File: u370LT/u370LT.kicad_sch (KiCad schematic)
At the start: 0 parts

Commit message: Updated northbridge more
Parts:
- added U1: ~, Library:BGA-676_26x26_35.0x35.0mm, symbol Library:VT82C694X
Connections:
- new net: U1.A1 (GND), U1.A14 (GND), U1.A26 (GND), U1.AA19 (GND), U1.AA21 (GND), U1.AA6 (GND), U1.AA8 (GND), U1.AB12 (GND), U1.AB15 (GND), U1.AB24 (GND), U1.AB25 (GND), U1.AC4 (GND), U1.AD18 (GND), U1.AD22 (GND), U1.AD9 (GND), U1.AE23 (GND), U1.AF1 (GND), U1.AF13 (GND), U1.AF26 (GND), U1.C18 (GND), U1.C22 (GND), U1.C5 (GND), U1.C9 (GND), U1.E12 (GND), U1.E15 (GND), U1.E24 (GND), U1.E3 (GND), U1.F19 (GND), U1.F21 (GND), U1.F6 (GND), U1.F8 (GND), U1.H21 (GND), U1.H6 (GND), U1.J24 (GND), U1.J3 (GND), U1.K1 (GND), U1.K7 (GND), U1.L12 (GND), U1.L15 (GND), U1.M11 (GND), U1.M13 (GND), U1.M14 (GND), U1.M16 (GND), U1.N12 (GND), U1.N13 (GND), U1.N14 (GND), U1.N15 (GND), U1.N24 (GND), U1.N7 (GND), U1.P12 (GND), U1.P13 (GND), U1.P14 (GND), U1.P15 (GND), U1.P22 (GND), U1.P26 (GND), U1.P3 (GND), U1.P7 (GND), U1.R11 (GND), U1.R13 (GND), U1.R14 (GND), U1.R16 (GND), U1.R22 (GND), U1.T12 (GND), U1.T15 (GND), U1.U6 (GND), U1.V24 (GND), U1.Y3 (GND), U1.Y6 (GND), U1.Y7 (GND), U1.Y8 (GND)
- new net: U1.AA18 (VCC), U1.AA20 (VCC), U1.AA9 (VCC), U1.AE26 (VCC), U1.AF14 (VCC), U1.B1 (VCC), U1.C2 (VCC), U1.F18 (VCC), U1.F20 (VCC), U1.F7 (VCC), U1.F9 (VCC), U1.G21 (VCC), U1.G6 (VCC), U1.J21 (VCC), U1.J6 (VCC), U1.L11 (VCC), U1.L13 (VCC), U1.L14 (VCC), U1.L16 (VCC), U1.M12 (VCC), U1.M15 (VCC), U1.N11 (VCC), U1.N16 (VCC), U1.N26 (VCC), U1.P11 (VCC), U1.P16 (VCC), U1.R12 (VCC), U1.R15 (VCC), U1.T11 (VCC), U1.T13 (VCC), U1.T14 (VCC), U1.T16 (VCC), U1.V21 (VCC)
- new net: U1.AA3 (VCCQ), U1.AA7 (VCCQ), U1.L6 (VCCQ), U1.L7 (VCCQ), U1.R3 (VCCQ), U1.R6 (VCCQ), U1.R7 (VCCQ)
- new net: U1.AD4 (VCCQQ), U1.W6 (VCCQ)
- new net: U1.L4 (ST0), U1.M4 (ST2)
- new net: U1.M21 (GNDA), U1.M22 (GNDA), U1.U7 (GNDA), U1.W21 (GNDA)
- new net: U1.N21 (VCCA), U1.N22 (VCCA), U1.V6 (VCCA), U1.Y21 (VCCA)

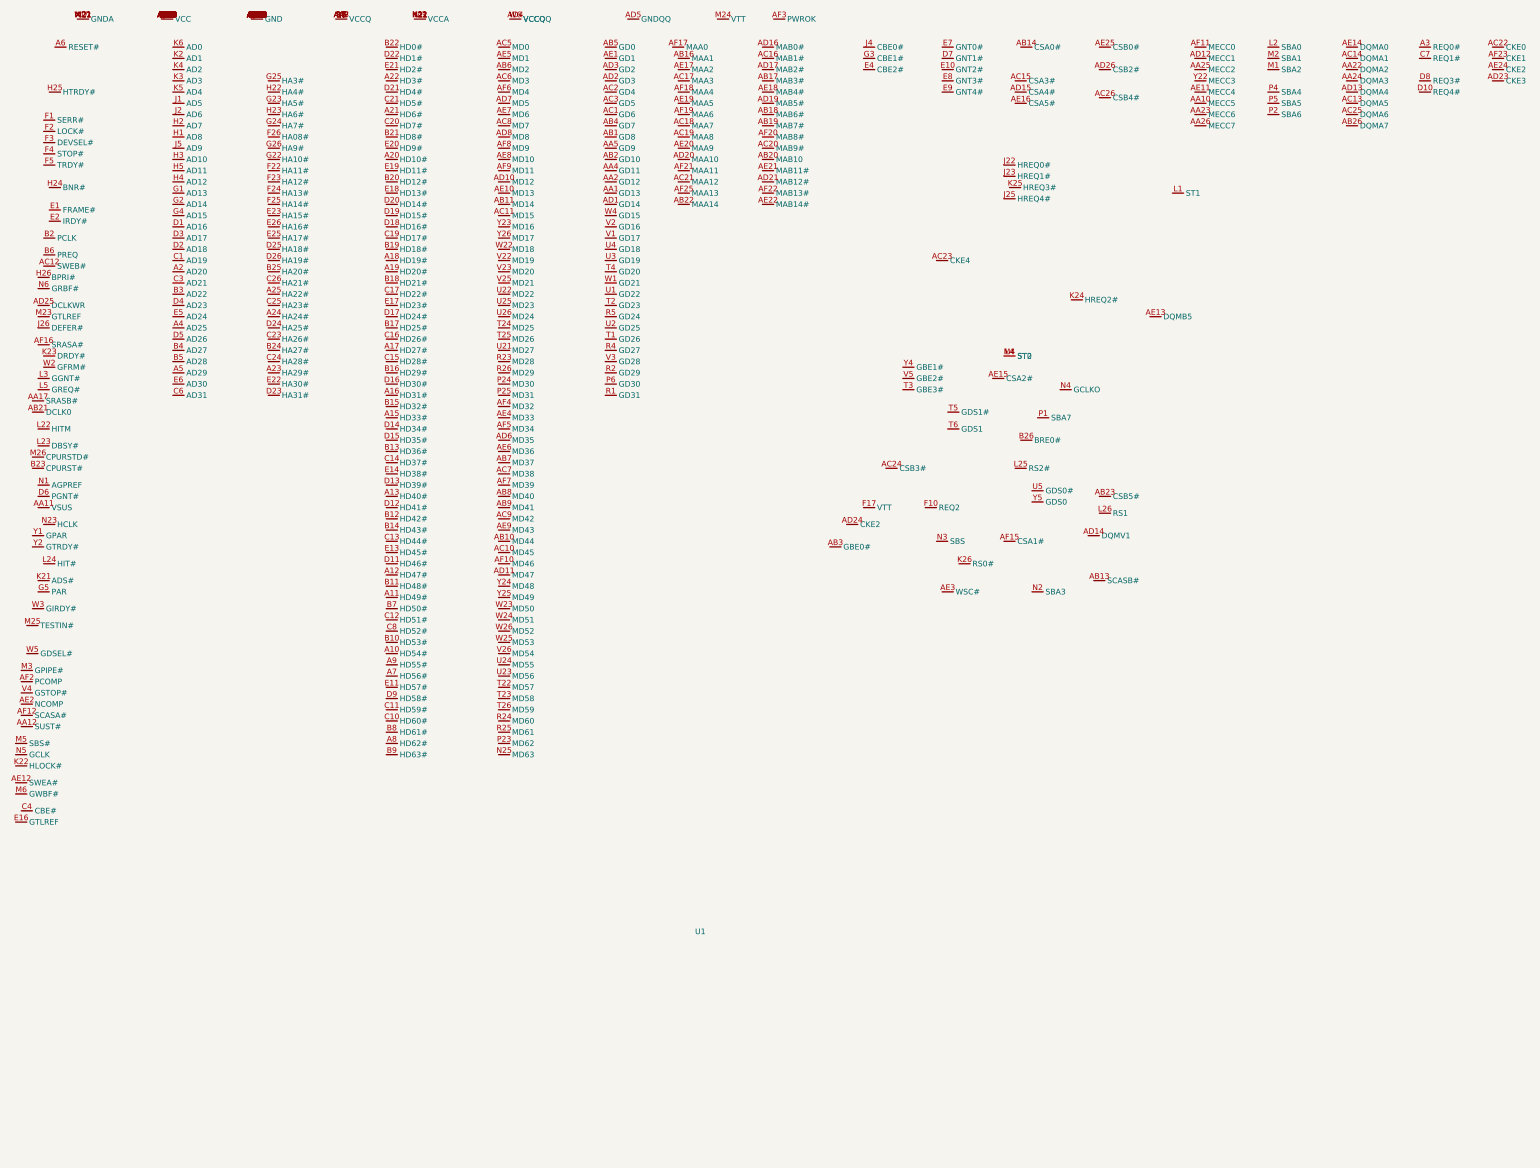
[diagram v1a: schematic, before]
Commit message: NB fixed up, SB started
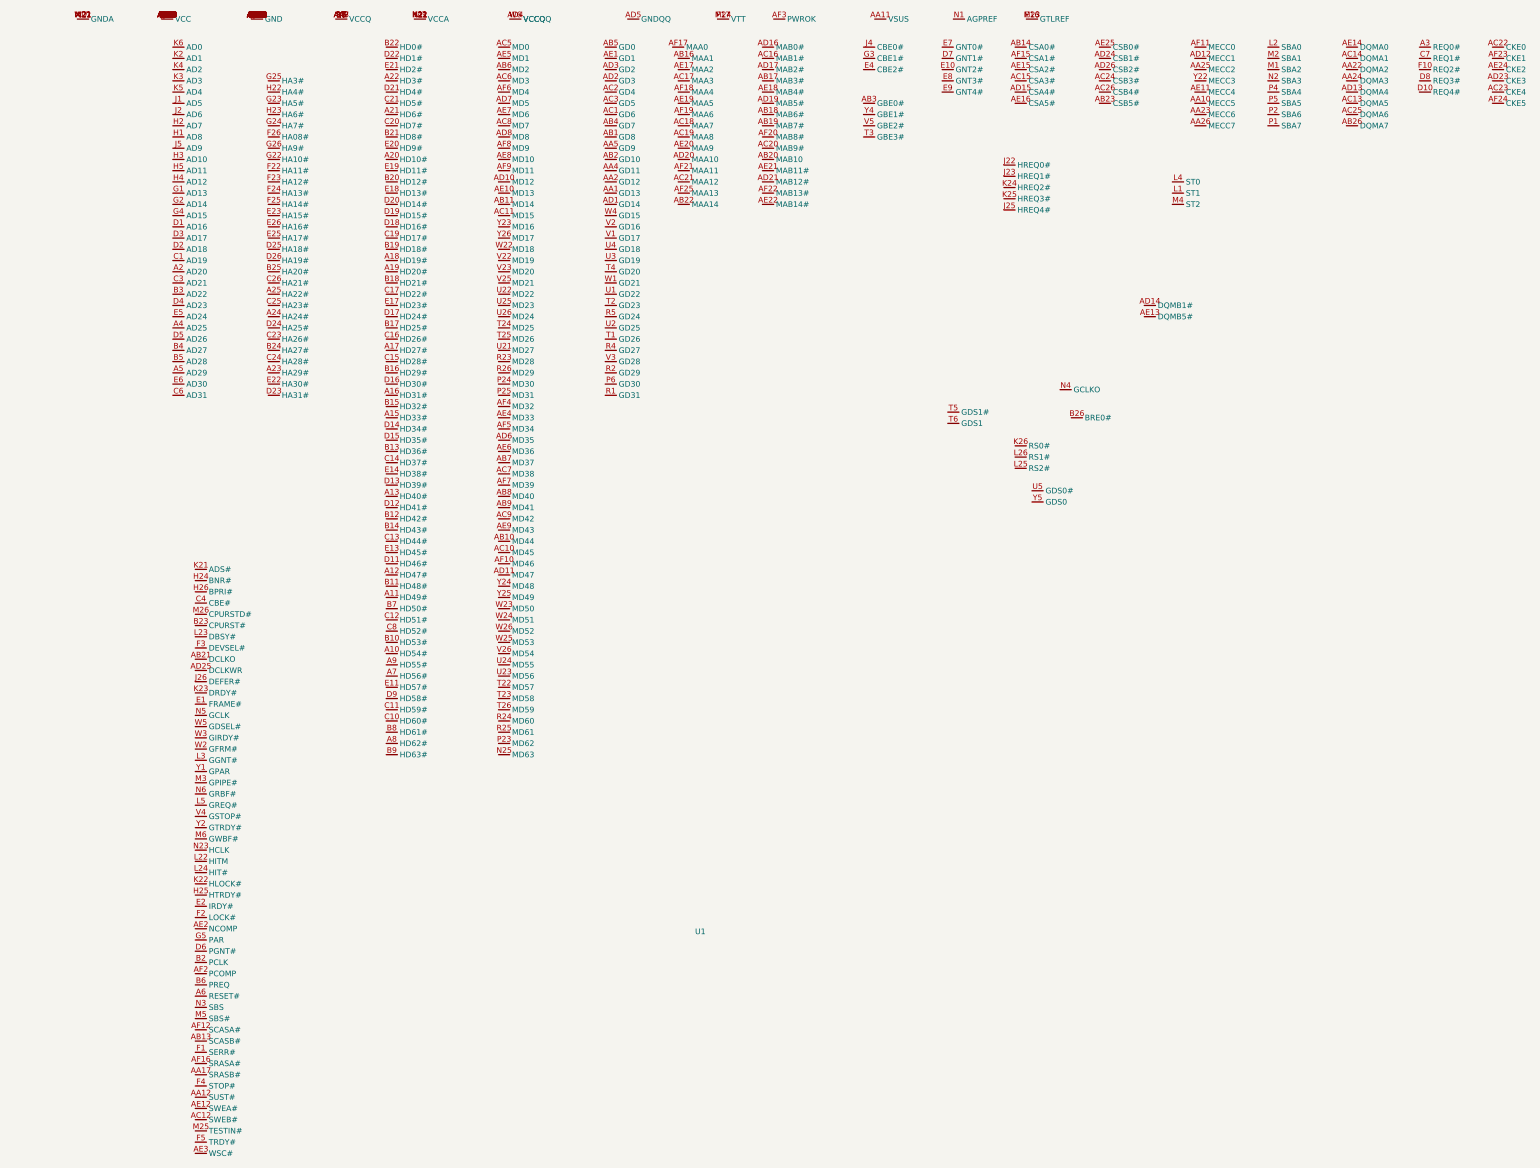
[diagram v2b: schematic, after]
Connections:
- net at U1.E16 (GTLREF): now also U1.M23 (GTLREF)
- net at U1.F17 (VTT): now also U1.M24 (VTT)
- net at U1.L4 (ST0): no longer U1.M4 (ST2)
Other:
- moved on the sheet: U1
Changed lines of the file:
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@@
 		(pin "U24"
+		)
+		(pin "AF24"
 		)
 		(instances
